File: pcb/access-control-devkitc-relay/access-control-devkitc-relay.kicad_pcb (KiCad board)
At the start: 2 copper layers, 24.6 x 57.5 mm, 15 parts, among them K1 G5LE-1

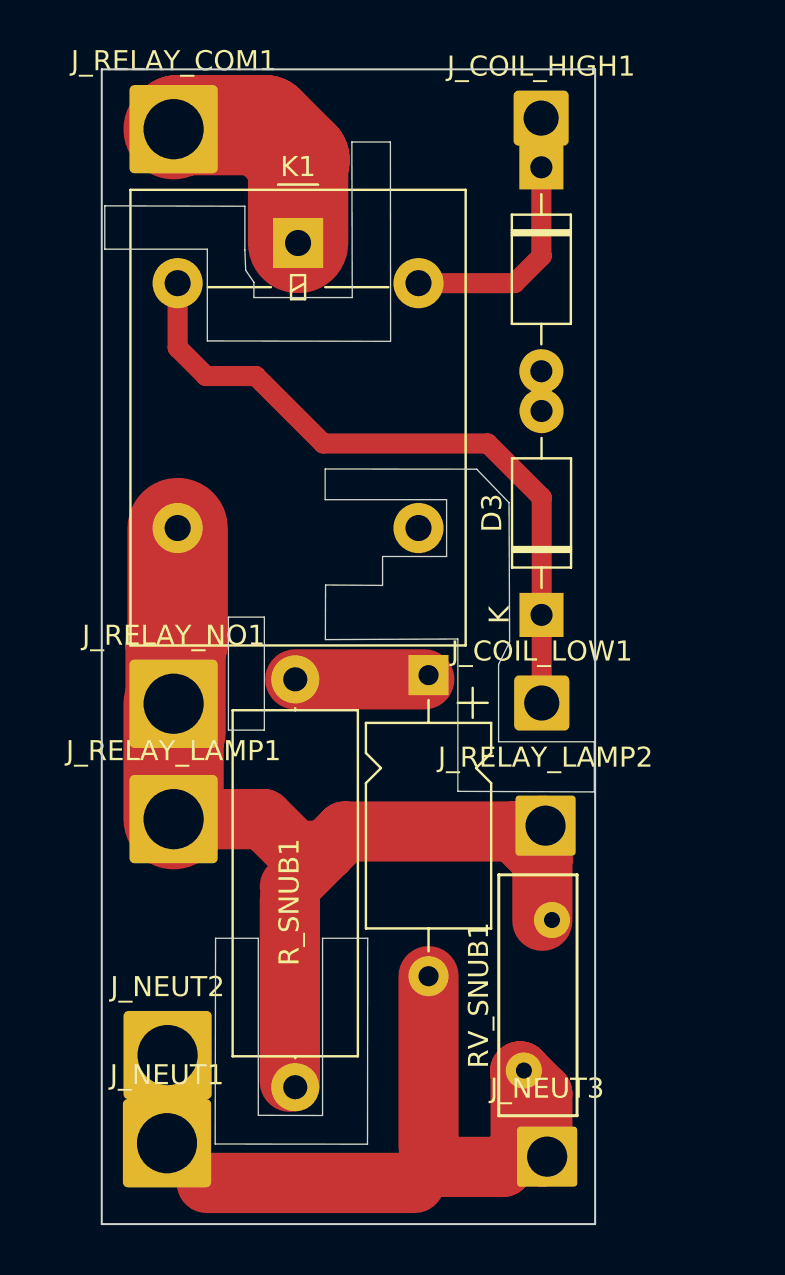
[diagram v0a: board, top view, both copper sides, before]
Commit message: Final changes pre manufacture
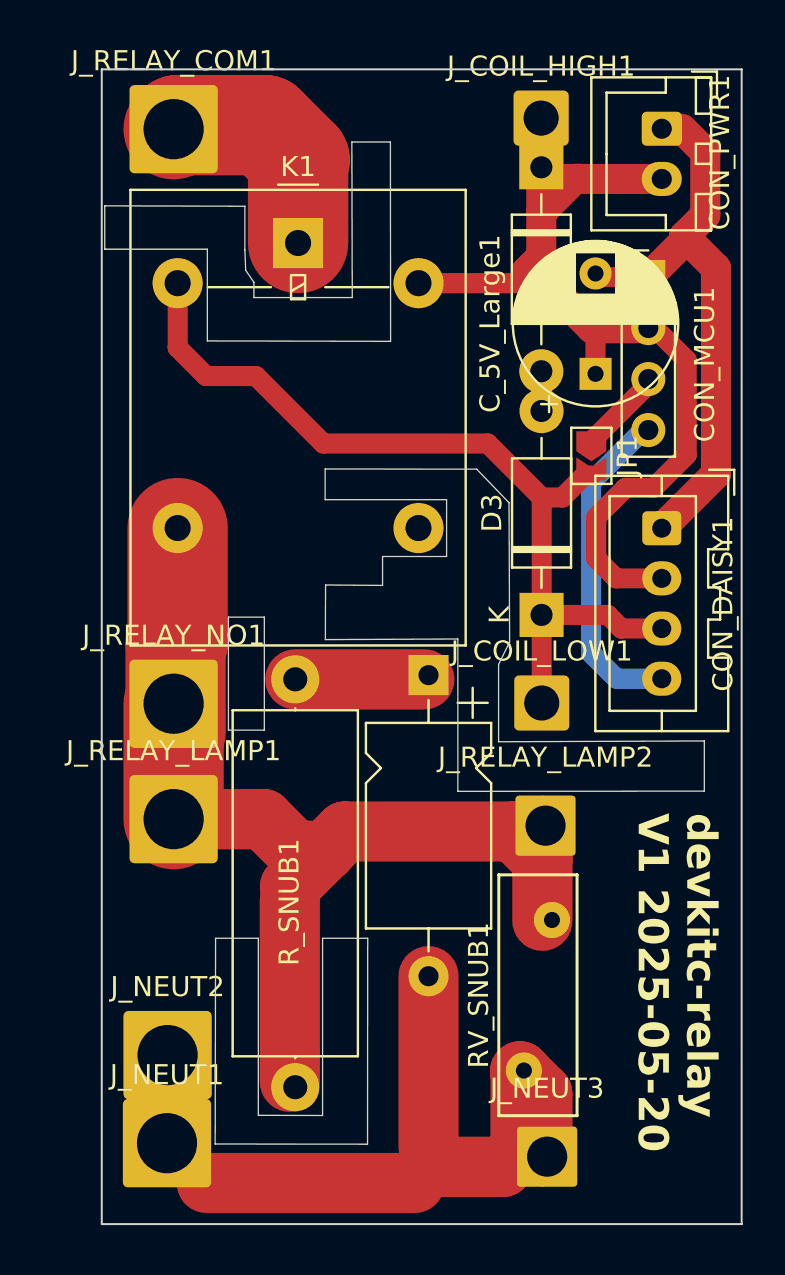
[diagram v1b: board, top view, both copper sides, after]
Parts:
- added CON_DAISY1: Conn_01x04_Socket, Connector_JST:JST_XA_B04B-XASK-1_1x04_P2.50mm_Vertical, F.Cu at (27.0, 22.7)
- added CON_MCU1: Conn_01x04_Socket, Connector_PinHeader_2.54mm:PinHeader_1x04_P2.54mm_Vertical, F.Cu at (26.3, 10.2)
- added CON_PWR1: Conn_01x02_Socket, Connector_JST:JST_XH_B2B-XH-A_1x02_P2.50mm_Vertical, F.Cu at (27.0, 2.80)
- added C_5V_Large1: 1000uf, Capacitor_THT:CP_Radial_D8.0mm_P5.00mm, F.Cu at (23.7, 15.0)
- added JP1: SolderJumper_2_Open, Jumper:SolderJumper-2_P1.3mm_Open_TrianglePad1.0x1.5mm, F.Cu at (23.5, 19.1)
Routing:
- net +5V: track 14.0 -> 51.3 mm
- net GND: track 0.00 -> 29.1 mm
- net Net-(CON_DAISY1-Pin_4): track 0.00 -> 16.2 mm
- net Net-(CON_DAISY1-Pin_3): track 34.7 -> 43.9 mm
- net Net-(CON_MCU1-Pin_3): track 0.00 -> 4.37 mm
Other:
- board size 24.6 x 57.5 mm -> 31.9 x 57.5 mm
- board text added: "devkitc-relay V1 2025-05-20"
